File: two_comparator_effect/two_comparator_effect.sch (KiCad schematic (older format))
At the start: 29 parts, among them J1 rca, J2 rca, J3 Barrel_Jack, Q1 2N3904, U1 LM339, U2 LM317

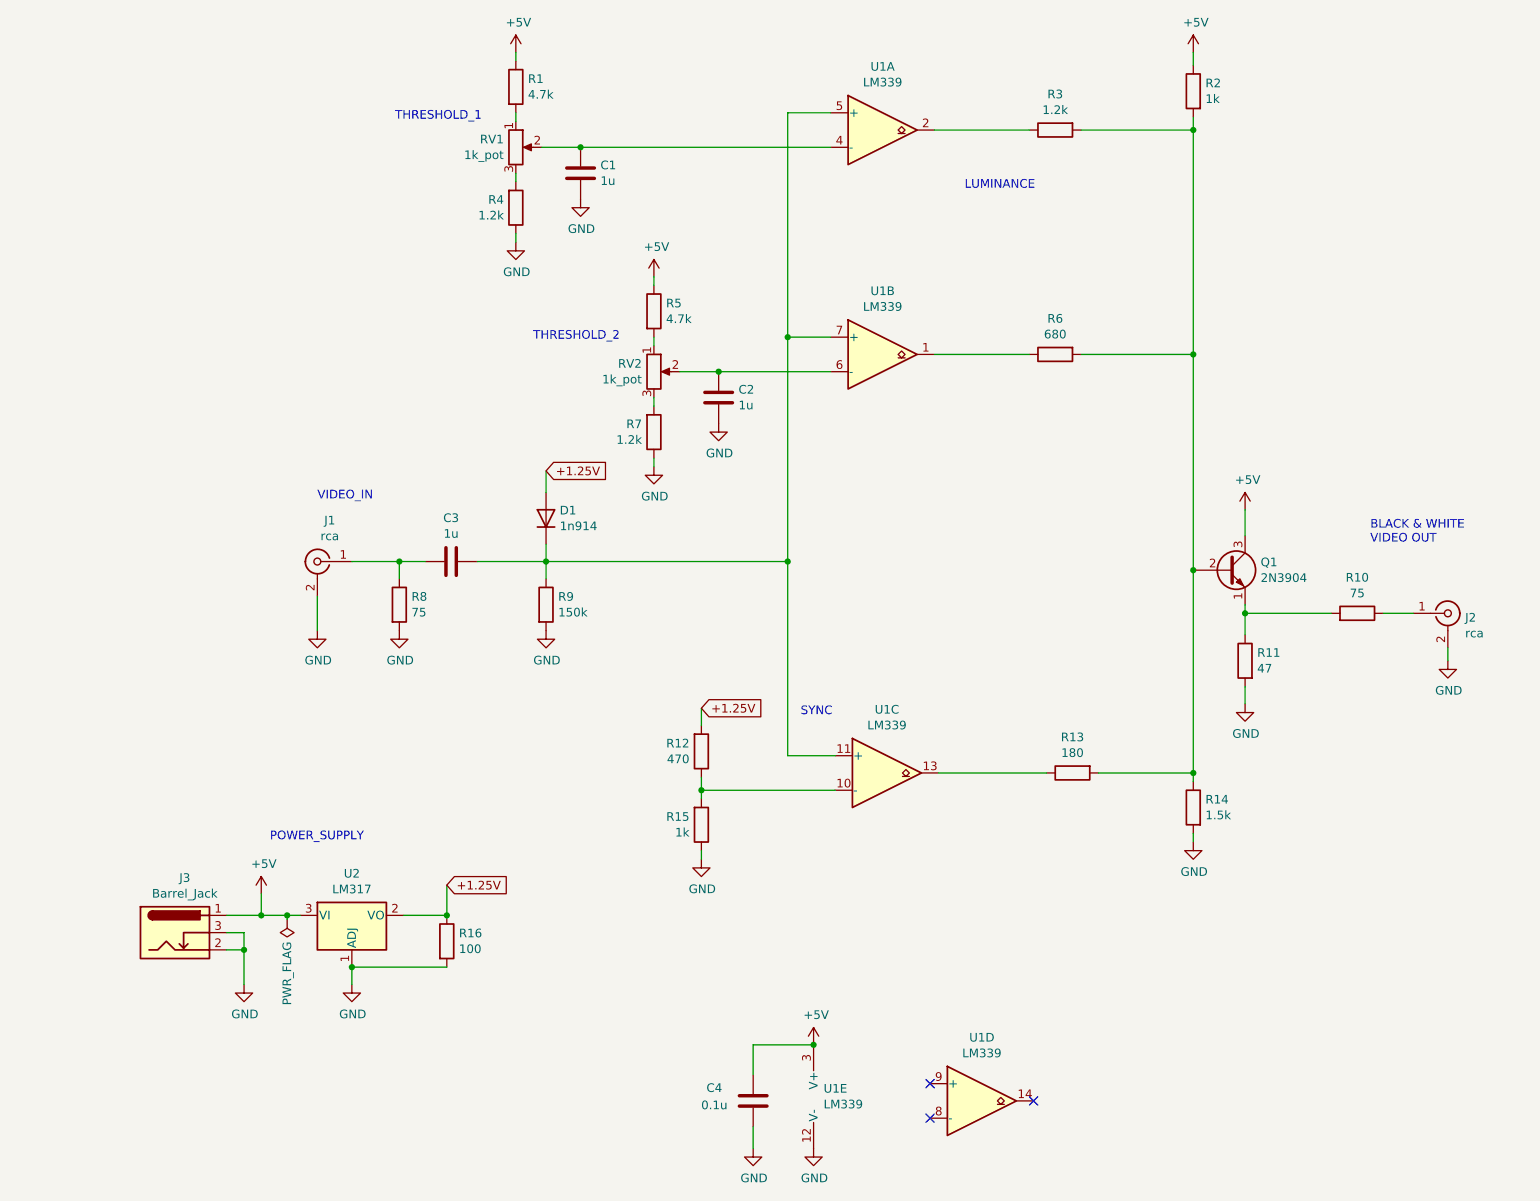
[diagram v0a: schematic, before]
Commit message: newest circuit revisions
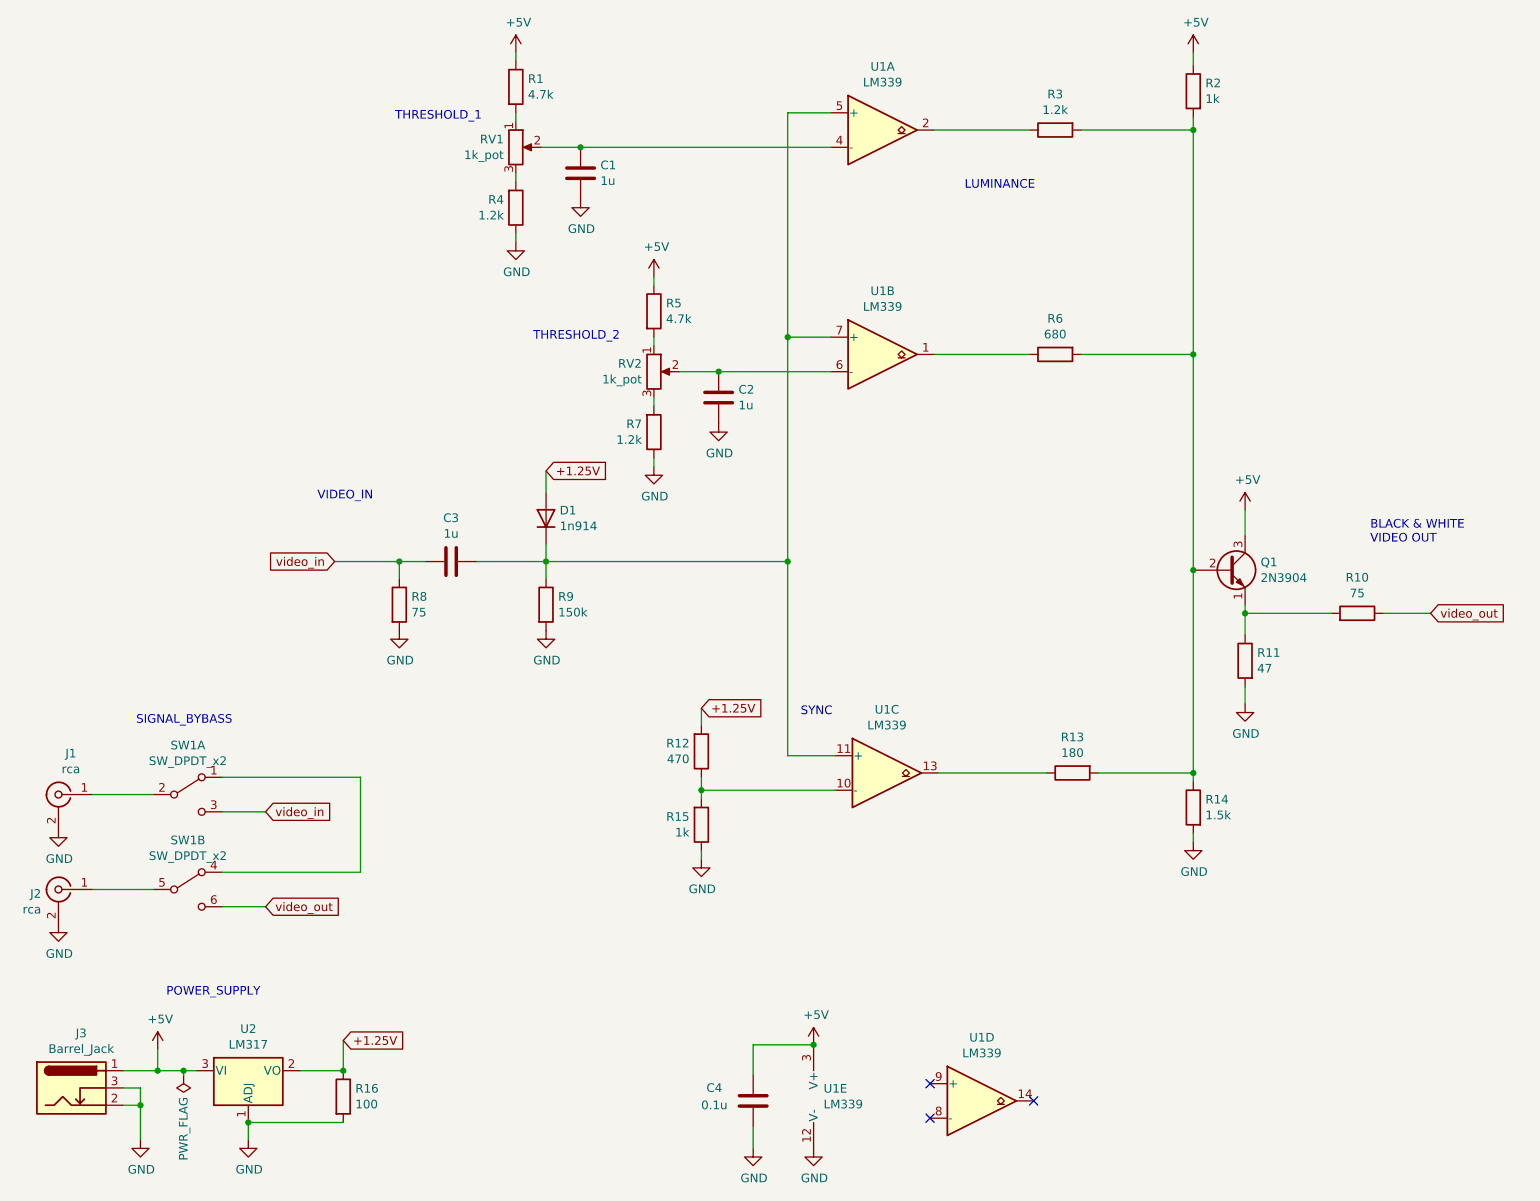
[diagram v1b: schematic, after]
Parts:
- added SW1: SW_DPDT_x2, lib:dpdt_mini_toggle_switch_tayda, symbol Switch:SW_DPDT_x2
- J1, J2: footprint lib_fp:tht_rca_vertical -> lib:tht_rca_vertical
- RV1, RV2: footprint lib_fp:Potentiometer_Vertical_Large -> lib:Potentiometer_Vertical_Large
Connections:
- net video_in: now reaches C3.2, R8.1
- net video_in: now also SW1.3 (C); no longer J1.1 (In)
- net at J2.1 (In): now also SW1.5 (B); no longer R10.1
- new net: J1.1 (In), SW1.2 (B)
- new net: SW1.1 (A), SW1.4 (A)
- new net video_out: R10.1, SW1.6 (C)
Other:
- note added: "SIGNAL_BYBASS"
- moved on the sheet: J1, J2, J3, R16, U2
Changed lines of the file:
@@
 L Regulator_Linear:LM317_3PinPackage U2
 U 1 1 5EB5729E
-P 2550 6100
-F 0 "U2" H 2550 6342 50  0000 C CNN
-F 1 "LM317" H 2550 6251 50  0000 C CNN
-F 2 "Package_TO_SOT_THT:TO-92_HandSolder" H 2550 6325 50  0001 C CIN
-F 3 "http://www.ti.com/lit/ds/snvs775k/snvs775k.pdf" H 2550 6100 50  0001 C CNN
-	1    2550 6100
+P 1950 7000
+F 0 "U2" H 1950 7242 50  0000 C CNN
+F 1 "LM317" H 1950 7151 50  0000 C CNN
+F 2 "Package_TO_SOT_THT:TO-92_HandSolder" H 1950 7225 50  0001 C CIN
+F 3 "http://www.ti.com/lit/ds/snvs775k/snvs775k.pdf" H 1950 7000 50  0001 C CNN
+	1    1950 7000
 	1    0    0    -1
 $EndComp
@@
 L power:GND #PWR023
 U 1 1 5EB57A13
-P 2550 6500
-F 0 "#PWR023" H 2550 6250 50  0001 C CNN
-F 1 "GND" H 2555 6327 50  0000 C CNN
-F 2 "" H 2550 6500 50  0001 C CNN
-F 3 "" H 2550 6500 50  0001 C CNN
-	1    2550 6500
-	1    0    0    -1
-$EndComp
-Wire Wire Line
-	2550 6400 2550 6500
+P 1950 7400
+F 0 "#PWR023" H 1950 7150 50  0001 C CNN
+F 1 "GND" H 1955 7227 50  0000 C CNN
+F 2 "" H 1950 7400 50  0001 C CNN
+F 3 "" H 1950 7400 50  0001 C CNN
+	1    1950 7400
+	1    0    0    -1
+$EndComp
+Wire Wire Line
+	1950 7300 1950 7400
 $Comp
 L power:+5V #PWR019
 U 1 1 5EB58912
-P 2025 5975
-F 0 "#PWR019" H 2025 5825 50  0001 C CNN
-F 1 "+5V" H 2040 6148 50  0000 C CNN
-F 2 "" H 2025 5975 50  0001 C CNN
-F 3 "" H 2025 5975 50  0001 C CNN
-	1    2025 5975
-	1    0    0    -1
-$EndComp
-Wire Wire Line
-	2025 5975 2025 6100
-Wire Wire Line
-	2025 6100 2175 6100
-Text GLabel 3100 5925 2    50   Input ~ 0
+P 1425 6875
+F 0 "#PWR019" H 1425 6725 50  0001 C CNN
+F 1 "+5V" H 1440 7048 50  0000 C CNN
+F 2 "" H 1425 6875 50  0001 C CNN
+F 3 "" H 1425 6875 50  0001 C CNN
+	1    1425 6875
+	1    0    0    -1
+$EndComp
+Wire Wire Line
+	1425 6875 1425 7000
+Wire Wire Line
+	1425 7000 1575 7000
+Text GLabel 2500 6825 2    50   Input ~ 0
 +1.25V
 Wire Wire Line
-	2850 6100 3100 6100
-Wire Wire Line
-	3100 6100 3100 5925
+	2250 7000 2500 7000
+Wire Wire Line
+	2500 7000 2500 6825
 $Comp
 L Device:R R16
 U 1 1 5EB5929E
-P 3100 6250
-F 0 "R16" H 3170 6296 50  0000 L CNN
-F 1 "100" H 3170 6205 50  0000 L CNN
-F 2 "Resistor_THT:R_Axial_DIN0207_L6.3mm_D2.5mm_P7.62mm_Horizontal" V 3030 6250 50  0001 C CNN
-F 3 "~" H 3100 6250 50  0001 C CNN
-	1    3100 6250
-	1    0    0    -1
-$EndComp
-Connection ~ 3100 6100
-Wire Wire Line
-	3100 6400 2550 6400
-Connection ~ 2550 6400
+P 2500 7150
+F 0 "R16" H 2570 7196 50  0000 L CNN
+F 1 "100" H 2570 7105 50  0000 L CNN
+F 2 "Resistor_THT:R_Axial_DIN0207_L6.3mm_D2.5mm_P7.62mm_Horizontal" V 2430 7150 50  0001 C CNN
+F 3 "~" H 2500 7150 50  0001 C CNN
+	1    2500 7150
+	1    0    0    -1
+$EndComp
+Connection ~ 2500 7000
+Wire Wire Line
+	2500 7300 1950 7300
+Connection ~ 1950 7300
 $Comp
 L power:GND #PWR013
 U 1 1 5EB5A54D
-P 2350 4450
-F 0 "#PWR013" H 2350 4200 50  0001 C CNN
-F 1 "GND" H 2355 4277 50  0000 C CNN
-F 2 "" H 2350 4450 50  0001 C CNN
-F 3 "" H 2350 4450 50  0001 C CNN
-	1    2350 4450
+P 850 5600
+F 0 "#PWR013" H 850 5350 50  0001 C CNN
+F 1 "GND" H 855 5427 50  0000 C CNN
+F 2 "" H 850 5600 50  0001 C CNN
+F 3 "" H 850 5600 50  0001 C CNN
+	1    850  5600
 	1    0    0    -1
 $EndComp
@@
 $EndComp
 Wire Wire Line
-	2550 4050 2825 4050
-Wire Wire Line
-	2350 4250 2350 4450
-Wire Wire Line
 	2825 4150 2825 4050
-Connection ~ 2825 4050
-Wire Wire Line
-	2825 4050 2975 4050
 Wire Wire Line
 	3675 4050 3675 4150
@@
 F 0 "RV2" H 4230 2996 50  0000 R CNN
 F 1 "1k_pot" H 4230 2905 50  0000 R CNN
-F 2 "lib_fp:Potentiometer_Vertical_Large" H 4300 2950 50  0001 C CNN
+F 2 "lib:Potentiometer_Vertical_Large" H 4300 2950 50  0001 C CNN
 F 3 "~" H 4300 2950 50  0001 C CNN
 	1    4300 2950
@@
 L Connector:Conn_Coaxial J2
 U 1 1 5EBAE02B
-P 8900 4350
-F 0 "J2" H 9000 4325 50  0000 L CNN
-F 1 "rca" H 9000 4234 50  0000 L CNN
-F 2 "lib_fp:tht_rca_vertical" H 8900 4350 50  0001 C CNN
-F 3 " ~" H 8900 4350 50  0001 C CNN
-	1    8900 4350
-	1    0    0    -1
-$EndComp
-Wire Wire Line
-	8525 4350 8700 4350
+P 850 5950
+F 0 "J2" H 950 5925 50  0000 L CNN
+F 1 "rca" H 950 5834 50  0000 L CNN
+F 2 "lib:tht_rca_vertical" H 850 5950 50  0001 C CNN
+F 3 " ~" H 850 5950 50  0001 C CNN
+	1    850  5950
+	-1   0    0    -1
+$EndComp
 $Comp
 L power:GND #PWR016
 U 1 1 5EBB0C30
-P 8900 4625
-F 0 "#PWR016" H 8900 4375 50  0001 C CNN
-F 1 "GND" H 8905 4452 50  0000 C CNN
-F 2 "" H 8900 4625 50  0001 C CNN
-F 3 "" H 8900 4625 50  0001 C CNN
-	1    8900 4625
-	1    0    0    -1
-$EndComp
-Wire Wire Line
-	8900 4550 8900 4625
+P 850 6150
+F 0 "#PWR016" H 850 5900 50  0001 C CNN
+F 1 "GND" H 855 5977 50  0000 C CNN
+F 2 "" H 850 6150 50  0001 C CNN
+F 3 "" H 850 6150 50  0001 C CNN
+	1    850  6150
+	1    0    0    -1
+$EndComp
 Text Notes 2350 3700 0    50   ~ 0
 VIDEO_IN
@@
 F 0 "RV1" H 3430 1696 50  0000 R CNN
 F 1 "1k_pot" H 3430 1605 50  0000 R CNN
-F 2 "lib_fp:Potentiometer_Vertical_Large" H 3500 1650 50  0001 C CNN
+F 2 "lib:Potentiometer_Vertical_Large" H 3500 1650 50  0001 C CNN
 F 3 "~" H 3500 1650 50  0001 C CNN
 	1    3500 1650
@@
 L power:PWR_FLAG #FLG0101
 U 1 1 5EE5DD74
-P 2175 6125
-F 0 "#FLG0101" H 2175 6200 50  0001 C CNN
-F 1 "PWR_FLAG" V 2175 6252 50  0000 L CNN
-F 2 "" H 2175 6125 50  0001 C CNN
-F 3 "~" H 2175 6125 50  0001 C CNN
-	1    2175 6125
+P 1575 7025
+F 0 "#FLG0101" H 1575 7100 50  0001 C CNN
+F 1 "PWR_FLAG" V 1575 7152 50  0000 L CNN
+F 2 "" H 1575 7025 50  0001 C CNN
+F 3 "~" H 1575 7025 50  0001 C CNN
+	1    1575 7025
 	-1   0    0    1
 $EndComp
@@
 L Connector:Barrel_Jack_Switch J3
 U 1 1 5EE8590E
-P 1525 6200
-F 0 "J3" H 1582 6517 50  0000 C CNN
-F 1 "Barrel_Jack" H 1582 6426 50  0000 C CNN
-F 2 "Connector_BarrelJack:BarrelJack_Horizontal" H 1575 6160 50  0001 C CNN
-F 3 "~" H 1575 6160 50  0001 C CNN
-	1    1525 6200
+P 925 7100
+F 0 "J3" H 982 7417 50  0000 C CNN
+F 1 "Barrel_Jack" H 982 7326 50  0000 C CNN
+F 2 "Connector_BarrelJack:BarrelJack_Horizontal" H 975 7060 50  0001 C CNN
+F 3 "~" H 975 7060 50  0001 C CNN
+	1    925  7100
 	1    0    0    -1
 $EndComp
@@
 L power:GND #PWR024
 U 1 1 5EE88B2A
-P 1925 6500
-F 0 "#PWR024" H 1925 6250 50  0001 C CNN
-F 1 "GND" H 1930 6327 50  0000 C CNN
-F 2 "" H 1925 6500 50  0001 C CNN
-F 3 "" H 1925 6500 50  0001 C CNN
-	1    1925 6500
-	1    0    0    -1
-$EndComp
-Wire Wire Line
-	1825 6200 1925 6200
-Wire Wire Line
-	1925 6200 1925 6300
-Wire Wire Line
-	1825 6300 1925 6300
-Connection ~ 1925 6300
-Wire Wire Line
-	1925 6300 1925 6500
-Wire Wire Line
-	1825 6100 2025 6100
-Connection ~ 2025 6100
-Wire Wire Line
-	2175 6125 2175 6100
-Connection ~ 2175 6100
-Wire Wire Line
-	2175 6100 2250 6100
-Text Notes 2075 5675 0    50   ~ 0
+P 1325 7400
+F 0 "#PWR024" H 1325 7150 50  0001 C CNN
+F 1 "GND" H 1330 7227 50  0000 C CNN
+F 2 "" H 1325 7400 50  0001 C CNN
+F 3 "" H 1325 7400 50  0001 C CNN
+	1    1325 7400
+	1    0    0    -1
+$EndComp
+Wire Wire Line
+	1225 7100 1325 7100
+Wire Wire Line
+	1325 7100 1325 7200
+Wire Wire Line
+	1225 7200 1325 7200
+Connection ~ 1325 7200
+Wire Wire Line
+	1325 7200 1325 7400
+Wire Wire Line
+	1225 7000 1425 7000
+Connection ~ 1425 7000
+Wire Wire Line
+	1575 7025 1575 7000
+Connection ~ 1575 7000
+Wire Wire Line
+	1575 7000 1650 7000
+Text Notes 1475 6575 0    50   ~ 0
 POWER_SUPPLY
 $Comp
@@
 L Connector:Conn_Coaxial J1
 U 1 1 5EB59891
-P 2350 4050
-F 0 "J1" H 2278 4288 50  0000 C CNN
-F 1 "rca" H 2278 4197 50  0000 C CNN
-F 2 "lib_fp:tht_rca_vertical" H 2350 4050 50  0001 C CNN
-F 3 " ~" H 2350 4050 50  0001 C CNN
-	1    2350 4050
+P 850 5400
+F 0 "J1" H 778 5638 50  0000 C CNN
+F 1 "rca" H 778 5547 50  0000 C CNN
+F 2 "lib:tht_rca_vertical" H 850 5400 50  0001 C CNN
+F 3 " ~" H 850 5400 50  0001 C CNN
+	1    850  5400
 	-1   0    0    -1
 $EndComp
+$Comp
+L Switch:SW_DPDT_x2 SW1
+U 1 1 6173B2E6
+P 1600 5400
+F 0 "SW1" H 1600 5685 50  0000 C CNN
+F 1 "SW_DPDT_x2" H 1600 5594 50  0000 C CNN
+F 2 "lib:dpdt_mini_toggle_switch_tayda" H 1600 5400 50  0001 C CNN
+F 3 "~" H 1600 5400 50  0001 C CNN
+	1    1600 5400
+	1    0    0    -1
+$EndComp
+$Comp
+L Switch:SW_DPDT_x2 SW1
+U 2 1 6173BAD5
+P 1600 5950
+F 0 "SW1" H 1600 6235 50  0000 C CNN
+F 1 "SW_DPDT_x2" H 1600 6144 50  0000 C CNN
+F 2 "lib:dpdt_mini_toggle_switch_tayda" H 1600 5950 50  0001 C CNN
+F 3 "~" H 1600 5950 50  0001 C CNN
+	2    1600 5950
+	1    0    0    -1
+$EndComp
+Wire Wire Line
+	1050 5400 1400 5400
+Wire Wire Line
+	1050 5950 1400 5950
+Text GLabel 2050 5500 2    50   Input ~ 0
+video_in
+Text GLabel 2450 4050 0    50   Input ~ 0
+video_in
+Wire Wire Line
+	2450 4050 2825 4050
+Connection ~ 2825 4050
+Wire Wire Line
+	2825 4050 2975 4050
+Text GLabel 2050 6050 2    50   Input ~ 0
+video_out
+Wire Wire Line
+	2050 6050 1800 6050
+Wire Wire Line
+	1800 5500 2050 5500
+Wire Wire Line
+	1800 5300 2600 5300
+Wire Wire Line
+	2600 5300 2600 5850
+Wire Wire Line
+	2600 5850 1800 5850
+Text GLabel 8800 4350 2    50   Input ~ 0
+video_out
+Wire Wire Line
+	8525 4350 8800 4350
+Text Notes 1300 5000 0    50   ~ 0
+SIGNAL_BYBASS
 $EndSCHEMATC
